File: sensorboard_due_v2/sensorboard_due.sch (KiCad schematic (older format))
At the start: 20 parts, among them J2 I2C_SLAVE, J4 GPS_UBLOX_NEO6M, J5 Micro_SD_Card, U1 HSCDANN001BA2A3, U4 MS5805-02BA01

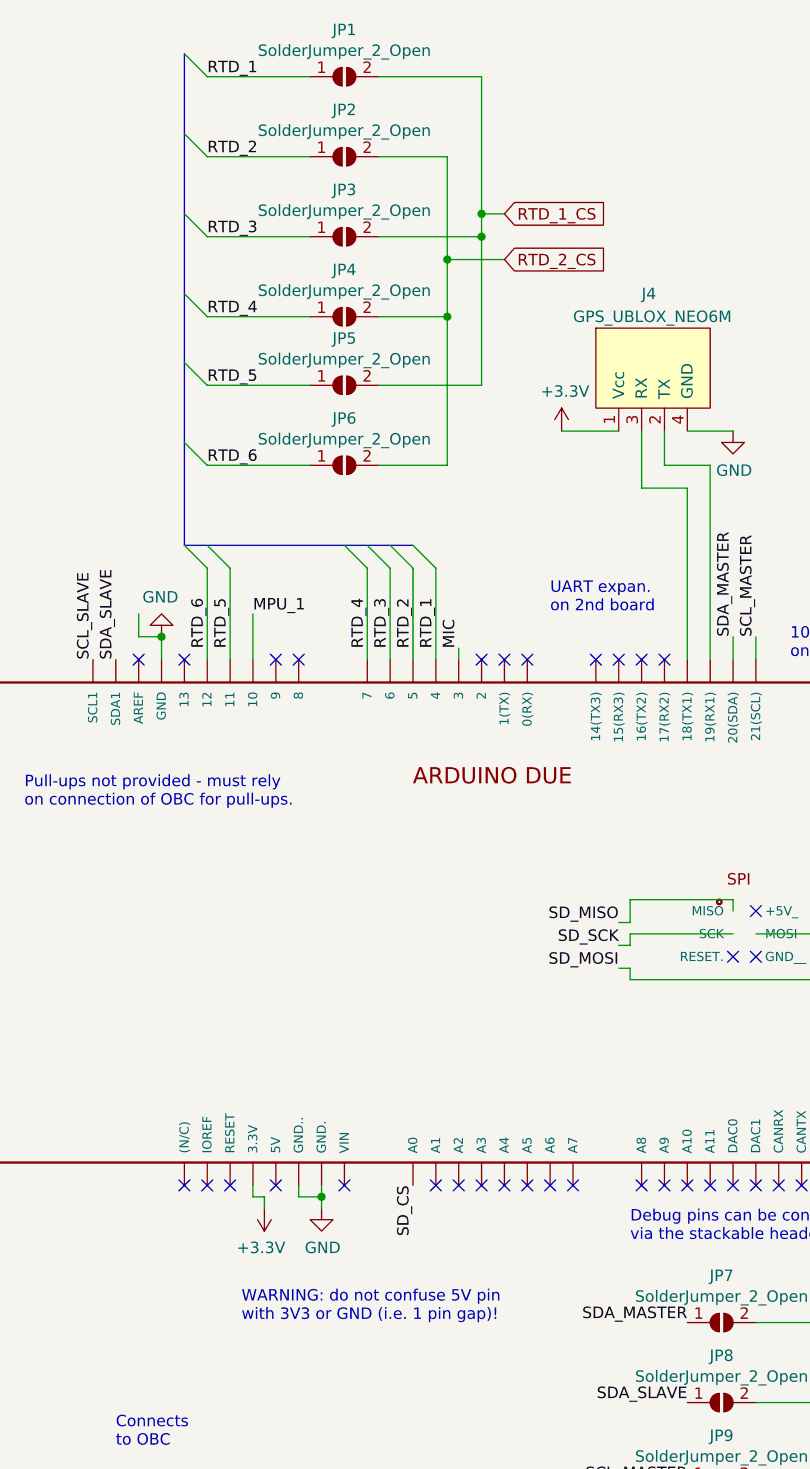
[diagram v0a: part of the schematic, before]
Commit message: incomplete pcb layout
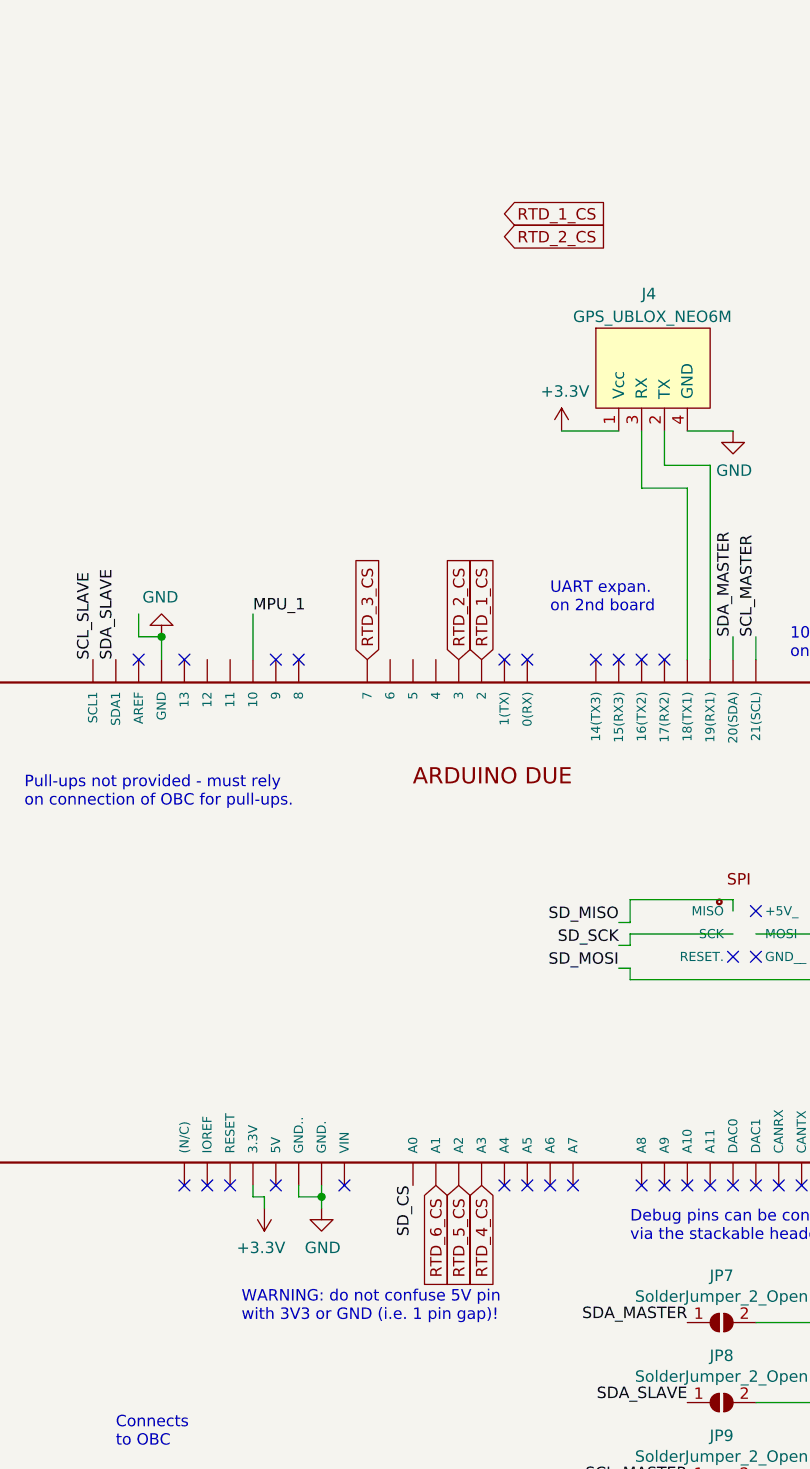
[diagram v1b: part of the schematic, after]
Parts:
- removed JP1, JP2, JP3, JP4, JP5, JP6: SolderJumper_2_Open, Jumper:SolderJumper-2_P1.3mm_Open_TrianglePad1.0x1.5mm, symbol Jumper:SolderJumper_2_Open
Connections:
- net MIC is gone; now on net RTD_2_CS: PCB1.3
- net RTD_1_CS: now also PCB1.2
- net RTD_6_CS: now reaches PCB1.A1
- net RTD_5_CS: now reaches PCB1.A2
- net RTD_4_CS: now reaches PCB1.A3
- net RTD_1: no longer names the net of PCB1.4
- net RTD_2: no longer names the net of PCB1.5
- net RTD_3: no longer names the net of PCB1.6
- net RTD_4 renamed RTD_3_CS
- net RTD_5: no longer names the net of PCB1.11
- net RTD_6: no longer names the net of PCB1.12
- no-connect marks 79 -> 75
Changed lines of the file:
@@
 NoConn ~ 2000 3650
 NoConn ~ 2100 3650
-NoConn ~ 2900 3650
 NoConn ~ 3000 3650
 NoConn ~ 3100 3650
@@
 Text GLabel 3000 1700 2    50   Input ~ 0
 RTD_1_CS
-Text GLabel 3000 1900 2    50   Input ~ 0
+Text GLabel 3000 1800 2    50   Input ~ 0
 RTD_2_CS
 Text Label 5600 6300 2    50   ~ 0
@@
 Text GLabel 5700 6500 2    50   Input ~ 0
 SCK
-$Comp
-L ARDUINO_DUE:ARDUINO_DUE_Shield_wSPI PCB1
-U 1 1 5E2A5E8E
-P 2900 4750
-F 0 "PCB1" H 2900 4750 50  0001 L BNN
-F 1 "ARDUINO_DUE" H 2900 4750 50  0001 L BNN
-F 2 "ARDUINO_DUE:ARDUINO_DUE_Shield_wSPI" H 2900 4750 50  0001 L BNN
-F 3 "" H 2900 4750 50  0001 C CNN
-	1    2900 4750
-	1    0    0    -1
-$EndComp
 Wire Wire Line
 	1900 3650 1900 3450
@@
 	1    0    0    -1
 $EndComp
-$Comp
-L Jumper:SolderJumper_2_Open JP1
-U 1 1 60BB0C16
-P 2300 1100
-F 0 "JP1" H 2300 1305 50  0000 C CNN
-F 1 "SolderJumper_2_Open" H 2300 1214 50  0000 C CNN
-F 2 "Jumper:SolderJumper-2_P1.3mm_Open_TrianglePad1.0x1.5mm" H 2300 1100 50  0001 C CNN
-F 3 "~" H 2300 1100 50  0001 C CNN
-	1    2300 1100
-	1    0    0    -1
-$EndComp
-$Comp
-L Jumper:SolderJumper_2_Open JP2
-U 1 1 60BB135A
-P 2300 1450
-F 0 "JP2" H 2300 1655 50  0000 C CNN
-F 1 "SolderJumper_2_Open" H 2300 1564 50  0000 C CNN
-F 2 "Jumper:SolderJumper-2_P1.3mm_Open_TrianglePad1.0x1.5mm" H 2300 1450 50  0001 C CNN
-F 3 "~" H 2300 1450 50  0001 C CNN
-	1    2300 1450
-	1    0    0    -1
-$EndComp
-$Comp
-L Jumper:SolderJumper_2_Open JP3
-U 1 1 60BBB104
-P 2300 1800
-F 0 "JP3" H 2300 2005 50  0000 C CNN
-F 1 "SolderJumper_2_Open" H 2300 1914 50  0000 C CNN
-F 2 "Jumper:SolderJumper-2_P1.3mm_Open_TrianglePad1.0x1.5mm" H 2300 1800 50  0001 C CNN
-F 3 "~" H 2300 1800 50  0001 C CNN
-	1    2300 1800
-	1    0    0    -1
-$EndComp
-$Comp
-L Jumper:SolderJumper_2_Open JP4
-U 1 1 60BBB10A
-P 2300 2150
-F 0 "JP4" H 2300 2355 50  0000 C CNN
-F 1 "SolderJumper_2_Open" H 2300 2264 50  0000 C CNN
-F 2 "Jumper:SolderJumper-2_P1.3mm_Open_TrianglePad1.0x1.5mm" H 2300 2150 50  0001 C CNN
-F 3 "~" H 2300 2150 50  0001 C CNN
-	1    2300 2150
-	1    0    0    -1
-$EndComp
-$Comp
-L Jumper:SolderJumper_2_Open JP5
-U 1 1 60BCBBB7
-P 2300 2450
-F 0 "JP5" H 2300 2655 50  0000 C CNN
-F 1 "SolderJumper_2_Open" H 2300 2564 50  0000 C CNN
-F 2 "Jumper:SolderJumper-2_P1.3mm_Open_TrianglePad1.0x1.5mm" H 2300 2450 50  0001 C CNN
-F 3 "~" H 2300 2450 50  0001 C CNN
-	1    2300 2450
-	1    0    0    -1
-$EndComp
-$Comp
-L Jumper:SolderJumper_2_Open JP6
-U 1 1 60BCBBBD
-P 2300 2800
-F 0 "JP6" H 2300 3005 50  0000 C CNN
-F 1 "SolderJumper_2_Open" H 2300 2914 50  0000 C CNN
-F 2 "Jumper:SolderJumper-2_P1.3mm_Open_TrianglePad1.0x1.5mm" H 2300 2800 50  0001 C CNN
-F 3 "~" H 2300 2800 50  0001 C CNN
-	1    2300 2800
-	1    0    0    -1
-$EndComp
-Entry Wire Line
-	2600 3150 2700 3250
-Entry Wire Line
-	2500 3150 2600 3250
-Entry Wire Line
-	2400 3150 2500 3250
-Entry Wire Line
-	2300 3150 2400 3250
-Wire Wire Line
-	2700 3650 2700 3250
-Wire Wire Line
-	2600 3250 2600 3650
-Wire Wire Line
-	2500 3650 2500 3250
-Wire Wire Line
-	2400 3650 2400 3250
-Entry Wire Line
-	1700 3150 1800 3250
-Entry Wire Line
-	1600 3150 1700 3250
-Wire Wire Line
-	1800 3250 1800 3650
-Wire Wire Line
-	1700 3650 1700 3250
-Text Label 2700 3600 1    50   ~ 0
-RTD_1
-Text Label 2600 3600 1    50   ~ 0
-RTD_2
-Text Label 2500 3600 1    50   ~ 0
-RTD_3
-Text Label 2400 3600 1    50   ~ 0
-RTD_4
-Text Label 1800 3600 1    50   ~ 0
-RTD_5
-Text Label 1700 3600 1    50   ~ 0
-RTD_6
-Wire Wire Line
-	3000 1700 2900 1700
-Wire Wire Line
-	2900 1700 2900 1100
-Wire Wire Line
-	2900 1700 2900 1800
-Connection ~ 2900 1700
-Wire Wire Line
-	2450 1100 2900 1100
-Wire Wire Line
-	2450 1800 2900 1800
-Connection ~ 2900 1800
-Wire Wire Line
-	2900 1800 2900 2450
-Wire Wire Line
-	2450 2450 2900 2450
-Wire Wire Line
-	2450 1450 2750 1450
-Wire Wire Line
-	2750 1450 2750 1900
-Wire Wire Line
-	2450 2800 2750 2800
-Wire Wire Line
-	2450 2150 2750 2150
-Connection ~ 2750 2150
-Wire Wire Line
-	2750 2150 2750 2800
-Wire Wire Line
-	3000 1900 2750 1900
-Connection ~ 2750 1900
-Wire Wire Line
-	2750 1900 2750 2150
-Entry Wire Line
-	1600 1000 1700 1100
-Entry Wire Line
-	1600 1350 1700 1450
-Entry Wire Line
-	1600 1700 1700 1800
-Entry Wire Line
-	1600 2050 1700 2150
-Entry Wire Line
-	1600 2350 1700 2450
-Entry Wire Line
-	1600 2700 1700 2800
-Wire Wire Line
-	2150 1100 1700 1100
-Wire Wire Line
-	2150 1450 1700 1450
-Wire Wire Line
-	2150 1800 1700 1800
-Wire Wire Line
-	2150 2450 1700 2450
-Wire Wire Line
-	2150 2800 1700 2800
-Text Label 1700 1100 0    50   ~ 0
-RTD_1
-Text Label 1700 1450 0    50   ~ 0
-RTD_2
-Text Label 1700 1800 0    50   ~ 0
-RTD_3
-Wire Wire Line
-	2150 2150 1700 2150
-Text Label 1700 2150 0    50   ~ 0
-RTD_4
-Text Label 1700 2450 0    50   ~ 0
-RTD_5
-Text Label 1700 2800 0    50   ~ 0
-RTD_6
 $Comp
 L power:GND #PWR0119
@@
 NoConn ~ 5100 4650
 NoConn ~ 5100 4750
-NoConn ~ 2700 5950
-NoConn ~ 2800 5950
-NoConn ~ 2900 5950
 NoConn ~ 3000 5950
 NoConn ~ 3100 5950
@@
 Wire Wire Line
 	9200 1650 8900 1650
-Text Label 2800 3600 1    50   ~ 0
-MIC
-Wire Wire Line
-	2800 3650 2800 3600
 Text Label 1200 3650 1    50   ~ 0
 SCL_SLAVE
@@
 Text Label 3800 7600 2    50   ~ 0
 SCL_SLAVE
-Wire Bus Line
-	1600 3150 2600 3150
-Wire Bus Line
-	1600 1000 1600 3150
+Text GLabel 2900 3650 1    50   Input ~ 0
+RTD_1_CS
+Text GLabel 2800 3650 1    50   Input ~ 0
+RTD_2_CS
+Text GLabel 2400 3650 1    50   Input ~ 0
+RTD_3_CS
+Text GLabel 2900 5950 3    50   Input ~ 0
+RTD_4_CS
+$Comp
+L ARDUINO_DUE:ARDUINO_DUE_Shield_wSPI PCB1
+U 1 1 5E2A5E8E
+P 2900 4750
+F 0 "PCB1" H 2900 4750 50  0001 L BNN
+F 1 "ARDUINO_DUE" H 2900 4750 50  0001 L BNN
+F 2 "ARDUINO_DUE:ARDUINO_DUE_Shield_wSPI" H 2900 4750 50  0001 L BNN
+F 3 "" H 2900 4750 50  0001 C CNN
+	1    2900 4750
+	1    0    0    -1
+$EndComp
+Text GLabel 2800 5950 3    50   Input ~ 0
+RTD_5_CS
+Text GLabel 2700 5950 3    50   Input ~ 0
+RTD_6_CS
 $EndSCHEMATC
